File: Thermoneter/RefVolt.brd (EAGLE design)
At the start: 15.2 x 16.5 mm, 8 parts

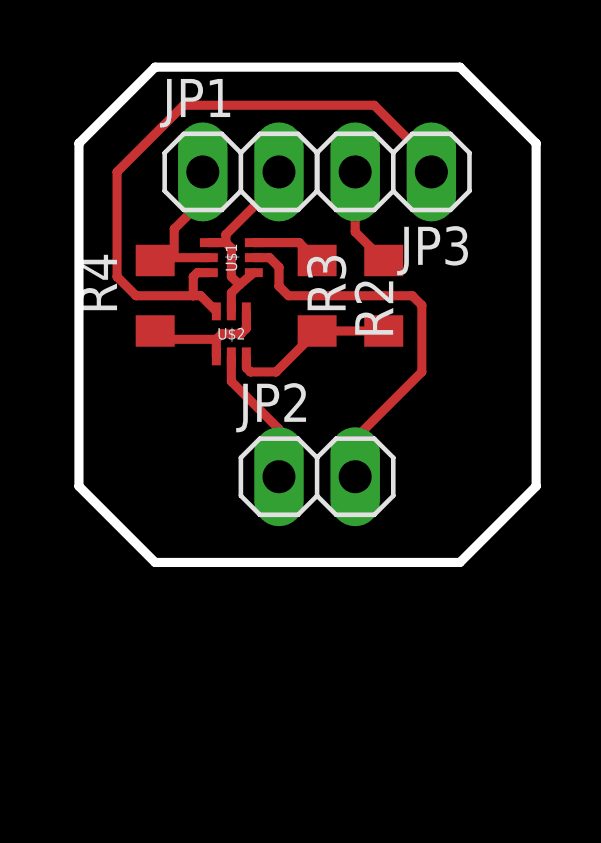
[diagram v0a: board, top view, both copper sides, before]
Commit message: _
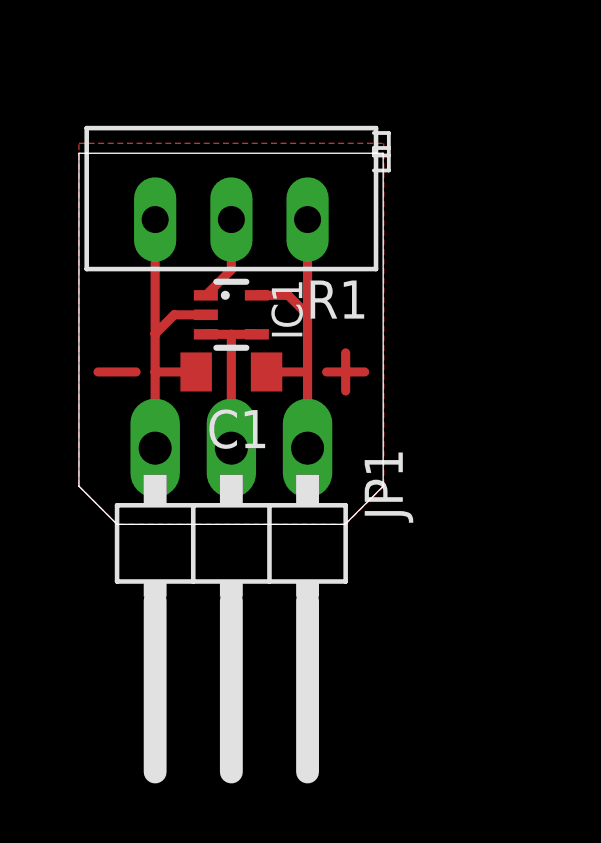
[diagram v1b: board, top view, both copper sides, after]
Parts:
- removed JP2, JP3: (no value), pinhead:1X02
- removed R2, R3, R4: 0, Namenlos:R0805
- removed U$1, U$2: FET-N/PNTZD3155C, Namenlos:SOT-563
- added C1: (no value), Namenlos:C0805
- added IC1: OP-AMP-1TSV521ICT, Namenlos:SC70-5L
- added R1: (no value), Namenlos:RJ9W
- JP1: device pinhead:1X02 -> pinhead:1X03/90
- moved JP1 13.0 mm to (3.81, -1.27), turned to 180 degrees
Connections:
- removed net N$10: R2.2, R3.1, U$2.3
- removed net N$11: JP1.1, R4.2, U$1.5
- removed net N$12: JP2.2, U$1.2
- removed net N$5: R4.1, U$2.1, U$2.4
- removed net N$7: JP1.2, U$1.1, U$1.4, U$2.5
- removed net N$8: JP2.1, U$2.2
- removed net N$9: R2.1, U$1.3
- new net N$1: IC1.3, IC1.4, JP1.2
- new net N$4: IC1.1, R1.W
- net GND: now also C1.2, IC1.2, JP1.3, R1.A; no longer JP3.1, U$1.6, U$2.6
- net VCC: now also C1.1, IC1.5, JP1.1, R1.B; no longer JP3.2, R3.2
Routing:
- net N$12: track 13.3 -> 0.00 mm
- net GND: track 21.0 -> 10.9 mm
- net VCC: track 3.35 -> 10.9 mm
- net N$7: track 7.19 -> 0.00 mm
- net N$10: track 5.59 -> 0.00 mm
- net N$1: track 0.00 -> 5.50 mm
- net N$11: track 5.08 -> 0.00 mm
- net N$8: track 4.67 -> 0.00 mm
- net N$5: track 4.44 -> 0.00 mm
- net N$4: track 0.00 -> 2.88 mm
- net N$9: track 2.35 -> 0.00 mm
- net N$2: track 0.00 -> 1.27 mm
- net N$6: track 0.00 -> 1.27 mm
- net N$3: track 0.00 -> 1.27 mm
- added copper zone on layer 1, net N$5
- removed copper zone on layer 1, net GND
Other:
- board size 15.2 x 16.5 mm -> 10.1 x 12.4 mm
